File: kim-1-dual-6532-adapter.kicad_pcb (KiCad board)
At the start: 2 copper layers, 75.3 x 68 mm, 14 parts, among them J2_1 6530_002_L, J2_2 6530_002_R, J3_1 6530_003_L, J3_2 6530_003_R, U1 27C64, U2 6532, U3 6532, U4 74LS138, U5 74LS00, U6 74LS04

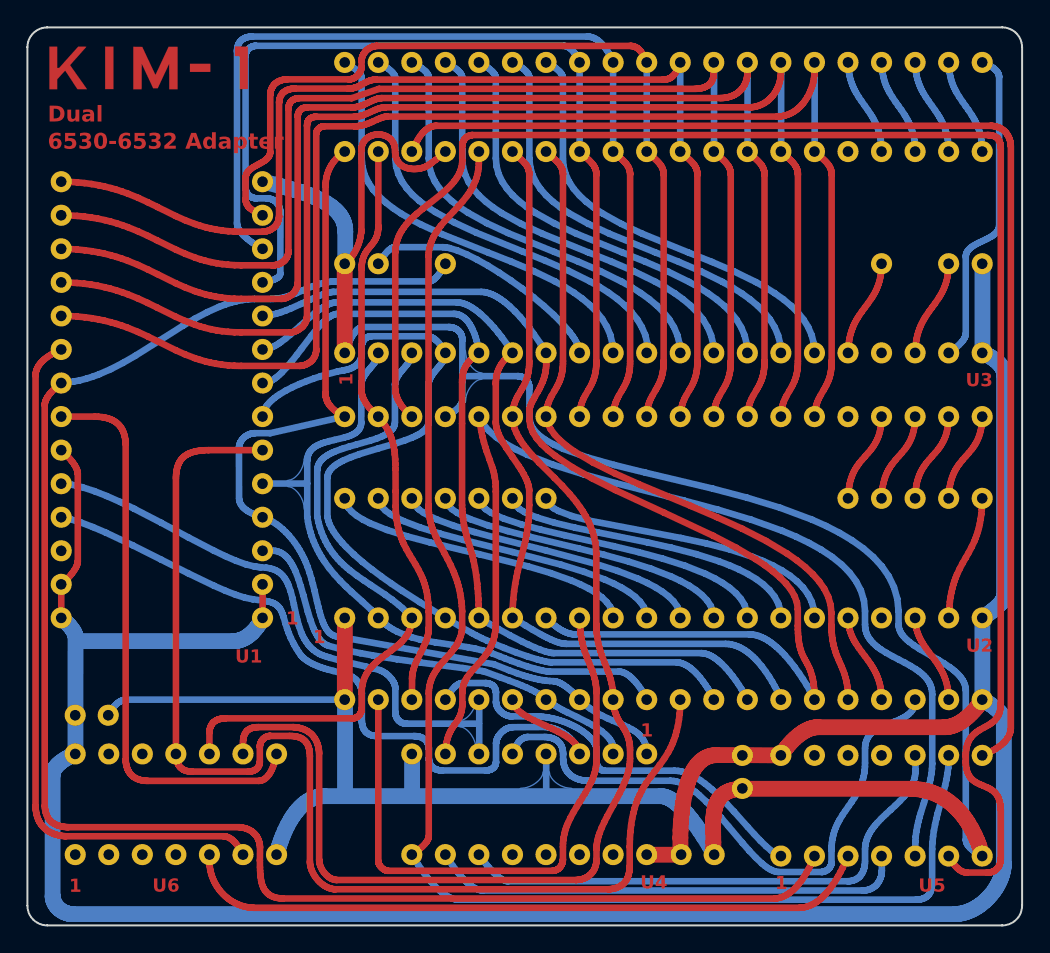
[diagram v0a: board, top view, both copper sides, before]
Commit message: Control ROM's OE with phi2
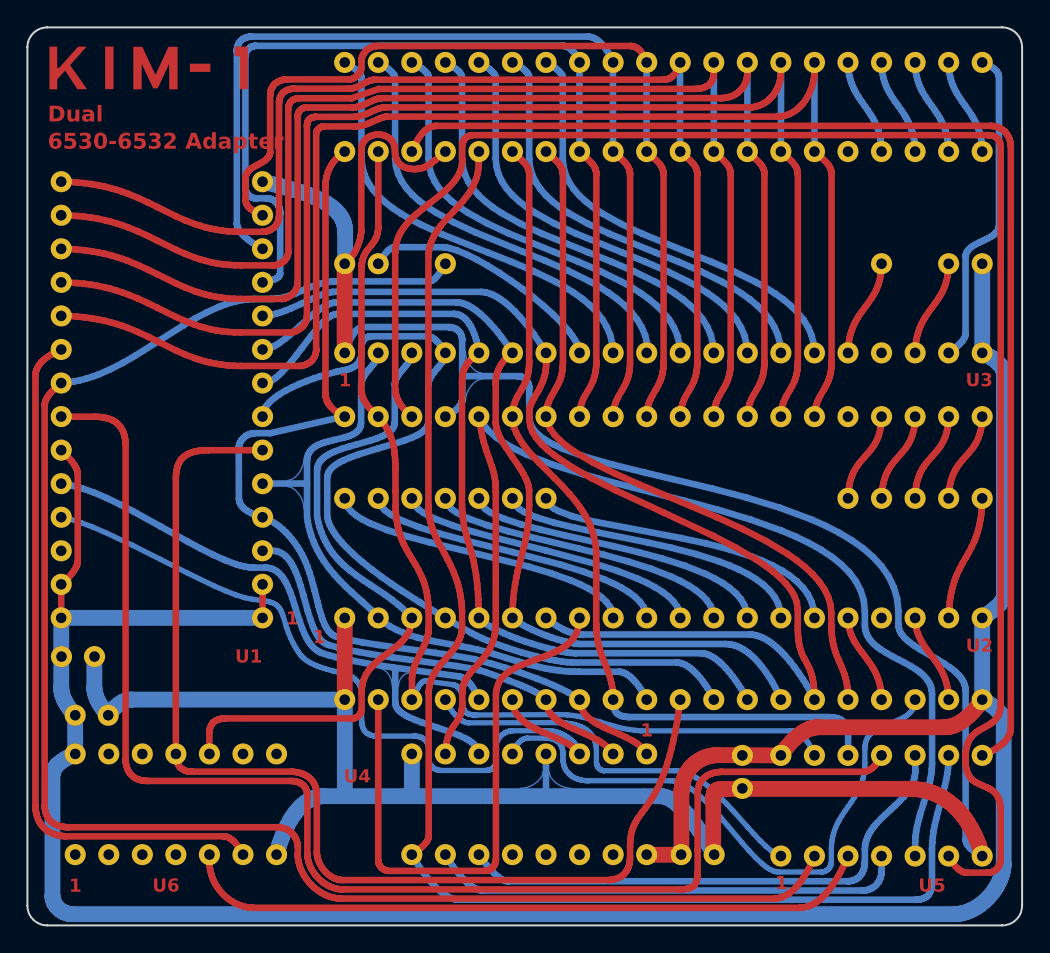
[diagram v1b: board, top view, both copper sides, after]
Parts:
- added C4: 100n, KIM-1_Library:C_Disc_D3.0mm_W2.0mm_P2.50mm, F.Cu at (35.6, 95.9)
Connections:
- U5 pad 11: unconnected-(U5-Pad11) -> Net-(U1-~{OE})
- U5 pad 12: unconnected-(U5-Pad12) -> /R/~{W}
- U5 pad 13: unconnected-(U5-Pad13) -> /Ø2
- U6 pad 8: Net-(U1-~{OE}) -> unconnected-(U6-Pad8)
- U6 pad 9: /R/~{W} -> unconnected-(U6-Pad9)
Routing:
- net Net-(U1-~{OE}): track 43.6 -> 103.0 mm
- net /Ø2: track 43.3 -> 77.3 mm
- net /R/~{W}: track 96.8 -> 65.6 mm
- net /A4: track 90.7 -> 84.3 mm
- net GND: track 217.3 -> 222.5 mm
- net /A9: track 44.4 -> 48.3 mm
- net /COLA: track 46.1 -> 43.8 mm
- net /K7: track 32.4 -> 31.1 mm
- net /K6: track 128.8 -> 128.0 mm
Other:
- rule pad_to_mask_clearance: 0.0508 -> 0
